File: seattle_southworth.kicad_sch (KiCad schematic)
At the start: 12 parts

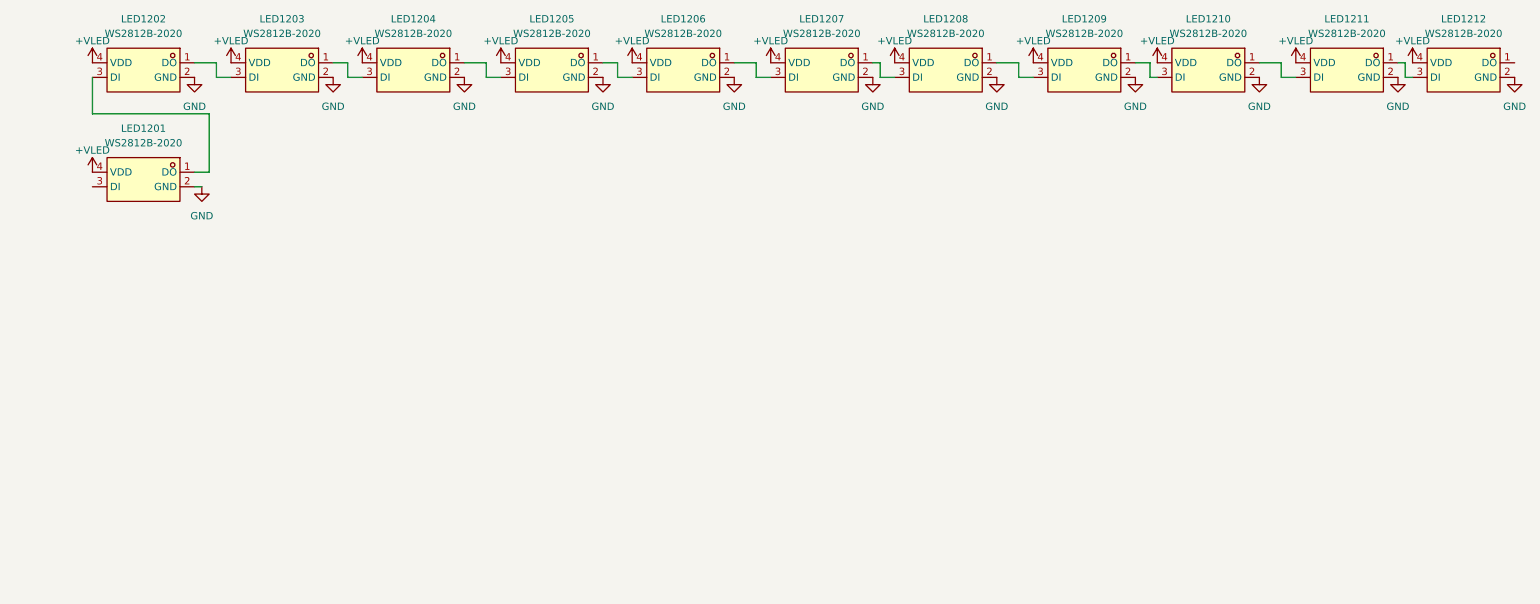
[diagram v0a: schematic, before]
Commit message: junction checkpoint
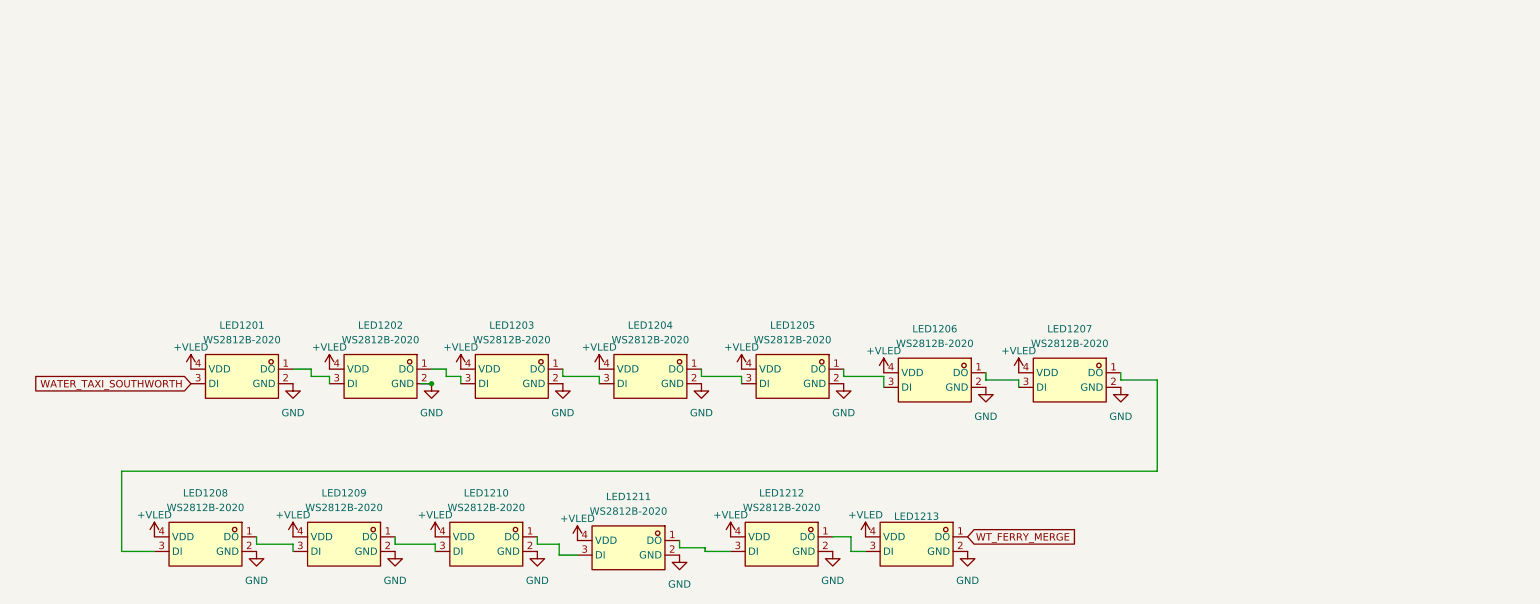
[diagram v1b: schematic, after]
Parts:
- added LED1213: WS2812B-2020, EasyEDA:LED-SMD_4P-L2.0-W2.0-TL_WS2812B-2020, symbol EasyEDA:WS2812B-2020
- renumbered LED1212 to LED1201, LED1211 to LED1202, LED1210 to LED1203, LED1209 to LED1204, LED1208 to LED1205, LED1207 to LED1206, LED1206 to LED1207, LED1205 to LED1208, LED1204 to LED1209, LED1203 to LED1210, LED1202 to LED1211, LED1201 to LED1212
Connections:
- net +VLED: now also LED1213.4 (VDD)
- net GND: now also LED1213.2 (GND)
- net at LED1208.1 (DO): now also LED1209.3 (DI); no longer LED1207.3 (DI)
- net at LED1208.3 (DI): now also LED1207.1 (DO); no longer LED1209.1 (DO)
- net at LED1202.1 (DO): now also LED1203.3 (DI); no longer LED1201.3 (DI)
- net at LED1202.3 (DI): now also LED1201.1 (DO); no longer LED1203.1 (DO)
- net at LED1212.1 (DO): now also LED1213.3 (DI); no longer LED1211.3 (DI)
- net at LED1212.3 (DI): now also LED1211.1 (DO)
- net at LED1204.1 (DO): now also LED1205.3 (DI); no longer LED1203.3 (DI)
- net at LED1204.3 (DI): now also LED1203.1 (DO); no longer LED1205.1 (DO)
- net at LED1210.1 (DO): now also LED1211.3 (DI); no longer LED1209.3 (DI)
- net at LED1206.1 (DO): now also LED1207.3 (DI); no longer LED1205.3 (DI)
- net at LED1206.3 (DI): now also LED1205.1 (DO); no longer LED1207.1 (DO)
- net at LED1210.3 (DI): now also LED1209.1 (DO); no longer LED1211.1 (DO)
- new net WATER_TAXI_SOUTHWORTH: LED1201.3 (DI)
- new net WT_FERRY_MERGE: LED1213.1 (DO)
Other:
- moved on the sheet: LED1201, LED1202, LED1203, LED1204, LED1205, LED1206, LED1207, LED1208, LED1209, LED1210, LED1211, LED1212

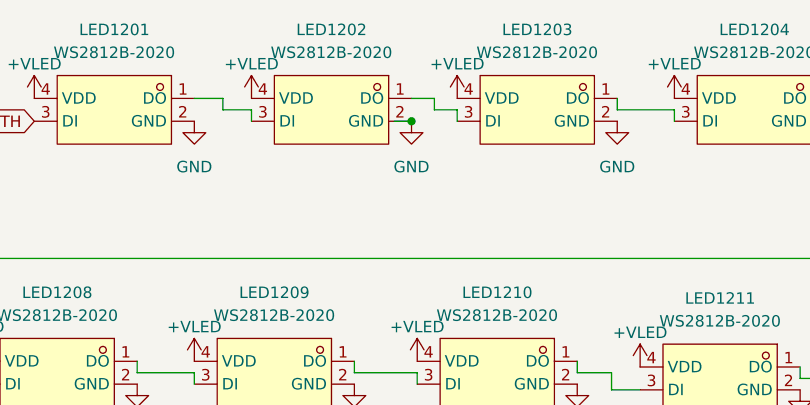
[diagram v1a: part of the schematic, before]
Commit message: rev-b validation run
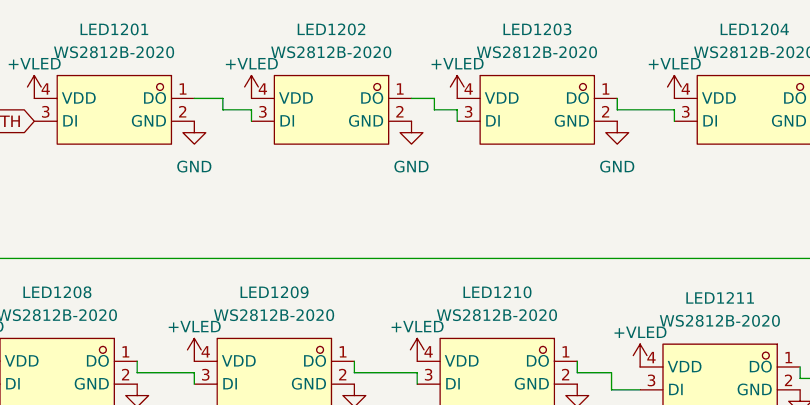
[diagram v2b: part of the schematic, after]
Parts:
- LED1201, LED1202, LED1203, LED1204, LED1205, LED1206, LED1207, LED1208, LED1209, LED1210, LED1211, LED1212, LED1213: LCSC Part C965555 -> C52917434
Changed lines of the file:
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@@
 	(generator_version "10.0")
 	(paper "A4")
-	(junction
-		(at 88.265 88.9)
-		(diameter 0)
-		(color 0 0 0 0)
-	)
 	(wire
 		(pts
@@
 	(wire
 		(pts
-			(xy 86.36 88.9) (xy 88.265 88.9)
-		)
-		(stroke
-			(width 0)
-			(type default)
-		)
-	)
-	(wire
-		(pts
 			(xy 190.5 88.265) (xy 190.5 89.535)
 		)
@@
 			)
 		)
-		(property "Datasheet" "https://lcsc.com/product-detail/Light-Emitting-Diodes-LED_Worldsemi-WS2812B-2020_C965555.html"
+		(property "Datasheet" "https://lcsc.com/product-detail/Light-Emitting-Diodes-LED_Worldsemi-WS2812B-2020_C52917434.html"
 			(at 181.61 128.27 0)
 			(hide yes)
@@
 			)
 		)
-		(property "LCSC Part" "C965555"
+		(property "LCSC Part" "C52917434"
 			(at 181.61 130.81 0)
 			(hide yes)
@@
 			)
 		)
-		(property "Datasheet" "https://lcsc.com/product-detail/Light-Emitting-Diodes-LED_Worldsemi-WS2812B-2020_C965555.html"
+		(property "Datasheet" "https://lcsc.com/product-detail/Light-Emitting-Diodes-LED_Worldsemi-WS2812B-2020_C52917434.html"
 			(at 57.785 128.27 0)
 			(hide yes)
@@
 			)
 		)
-		(property "LCSC Part" "C965555"
+		(property "LCSC Part" "C52917434"
 			(at 57.785 130.81 0)
 			(hide yes)
@@
 			)
 		)
-		(property "Datasheet" "https://lcsc.com/product-detail/Light-Emitting-Diodes-LED_Worldsemi-WS2812B-2020_C965555.html"
+		(property "Datasheet" "https://lcsc.com/product-detail/Light-Emitting-Diodes-LED_Worldsemi-WS2812B-2020_C52917434.html"
 			(at 88.265 99.06 0)
 			(hide yes)
@@
 			)
 		)
-		(property "LCSC Part" "C965555"
+		(property "LCSC Part" "C52917434"
 			(at 88.265 101.6 0)
 			(hide yes)
@@
 			)
 		)
-		(property "Datasheet" "https://lcsc.com/product-detail/Light-Emitting-Diodes-LED_Worldsemi-WS2812B-2020_C965555.html"
+		(property "Datasheet" "https://lcsc.com/product-detail/Light-Emitting-Diodes-LED_Worldsemi-WS2812B-2020_C52917434.html"
 			(at 158.115 128.27 0)
 			(hide yes)
@@
 			)
 		)
-		(property "LCSC Part" "C965555"
+		(property "LCSC Part" "C52917434"
 			(at 158.115 130.81 0)
 			(hide yes)
@@
 			)
 		)
-		(property "Datasheet" "https://lcsc.com/product-detail/Light-Emitting-Diodes-LED_Worldsemi-WS2812B-2020_C965555.html"
+		(property "Datasheet" "https://lcsc.com/product-detail/Light-Emitting-Diodes-LED_Worldsemi-WS2812B-2020_C52917434.html"
 			(at 135.255 99.06 0)
 			(hide yes)
@@
 			)
 		)
-		(property "LCSC Part" "C965555"
+		(property "LCSC Part" "C52917434"
 			(at 135.255 101.6 0)
 			(hide yes)
@@
 			)
 		)
-		(property "Datasheet" "https://lcsc.com/product-detail/Light-Emitting-Diodes-LED_Worldsemi-WS2812B-2020_C965555.html"
+		(property "Datasheet" "https://lcsc.com/product-detail/Light-Emitting-Diodes-LED_Worldsemi-WS2812B-2020_C52917434.html"
 			(at 81.915 128.27 0)
 			(hide yes)
@@
 			)
 		)
-		(property "LCSC Part" "C965555"
+		(property "LCSC Part" "C52917434"
 			(at 81.915 130.81 0)
 			(hide yes)
@@
 			)
 		)
-		(property "Datasheet" "https://lcsc.com/product-detail/Light-Emitting-Diodes-LED_Worldsemi-WS2812B-2020_C965555.html"
+		(property "Datasheet" "https://lcsc.com/product-detail/Light-Emitting-Diodes-LED_Worldsemi-WS2812B-2020_C52917434.html"
 			(at 64.135 99.06 0)
 			(hide yes)
@@
 			)
 		)
-		(property "LCSC Part" "C965555"
+		(property "LCSC Part" "C52917434"
 			(at 64.135 101.6 0)
 			(hide yes)
@@
 			)
 		)
-		(property "Datasheet" "https://lcsc.com/product-detail/Light-Emitting-Diodes-LED_Worldsemi-WS2812B-2020_C965555.html"
+		(property "Datasheet" "https://lcsc.com/product-detail/Light-Emitting-Diodes-LED_Worldsemi-WS2812B-2020_C52917434.html"
 			(at 184.785 99.695 0)
 			(hide yes)
@@
 			)
 		)
-		(property "LCSC Part" "C965555"
+		(property "LCSC Part" "C52917434"
 			(at 184.785 102.235 0)
 			(hide yes)
@@
 			)
 		)
-		(property "Datasheet" "https://lcsc.com/product-detail/Light-Emitting-Diodes-LED_Worldsemi-WS2812B-2020_C965555.html"
+		(property "Datasheet" "https://lcsc.com/product-detail/Light-Emitting-Diodes-LED_Worldsemi-WS2812B-2020_C52917434.html"
 			(at 208.28 99.695 0)
 			(hide yes)
@@
 			)
 		)
-		(property "LCSC Part" "C965555"
+		(property "LCSC Part" "C52917434"
 			(at 208.28 102.235 0)
 			(hide yes)
@@
 			)
 		)
-		(property "Datasheet" "https://lcsc.com/product-detail/Light-Emitting-Diodes-LED_Worldsemi-WS2812B-2020_C965555.html"
+		(property "Datasheet" "https://lcsc.com/product-detail/Light-Emitting-Diodes-LED_Worldsemi-WS2812B-2020_C52917434.html"
 			(at 106.68 128.27 0)
 			(hide yes)
@@
 			)
 		)
-		(property "LCSC Part" "C965555"
+		(property "LCSC Part" "C52917434"
 			(at 106.68 130.81 0)
 			(hide yes)
@@
 			)
 		)
-		(property "Datasheet" "https://lcsc.com/product-detail/Light-Emitting-Diodes-LED_Worldsemi-WS2812B-2020_C965555.html"
+		(property "Datasheet" "https://lcsc.com/product-detail/Light-Emitting-Diodes-LED_Worldsemi-WS2812B-2020_C52917434.html"
 			(at 111.125 99.06 0)
 			(hide yes)
@@
 			)
 		)
-		(property "LCSC Part" "C965555"
+		(property "LCSC Part" "C52917434"
 			(at 111.125 101.6 0)
 			(hide yes)
@@
 			)
 		)
-		(property "Datasheet" "https://lcsc.com/product-detail/Light-Emitting-Diodes-LED_Worldsemi-WS2812B-2020_C965555.html"
+		(property "Datasheet" "https://lcsc.com/product-detail/Light-Emitting-Diodes-LED_Worldsemi-WS2812B-2020_C52917434.html"
 			(at 131.445 128.905 0)
 			(hide yes)
@@
 			)
 		)
-		(property "LCSC Part" "C965555"
+		(property "LCSC Part" "C52917434"
 			(at 131.445 131.445 0)
 			(hide yes)
@@
 			)
 		)
-		(property "Datasheet" "https://lcsc.com/product-detail/Light-Emitting-Diodes-LED_Worldsemi-WS2812B-2020_C965555.html"
+		(property "Datasheet" "https://lcsc.com/product-detail/Light-Emitting-Diodes-LED_Worldsemi-WS2812B-2020_C52917434.html"
 			(at 160.02 99.06 0)
 			(hide yes)
@@
 			)
 		)
-		(property "LCSC Part" "C965555"
+		(property "LCSC Part" "C52917434"
 			(at 160.02 101.6 0)
 			(hide yes)
